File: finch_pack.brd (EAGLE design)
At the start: 14.6 x 28.3 mm, 5 parts

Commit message: board file
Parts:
- FHM-02PGR: device fujikura-fhm:FHM-02PG -> fujikura-fhm:FHM-02PGR
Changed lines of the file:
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@@
 </autorouter>
 <elements>
-<element name="FHM-02PGR" library="fujikura-fhm" package="FHM-02PG" value="FHM-02PGR" x="7.482109375" y="19.67463125" smashed="yes">
+<element name="FHM-02PGR" library="fujikura-fhm" package="FHM-02PGR" value="FHM-02PGR" x="7.482109375" y="19.67463125" smashed="yes">
 <attribute name="NAME" x="4.8442" y="16.611578125" size="0.254" layer="32" display="off"/>
 <attribute name="VALUE" x="5.80945625" y="17.18913125" size="0.4064" layer="21"/>

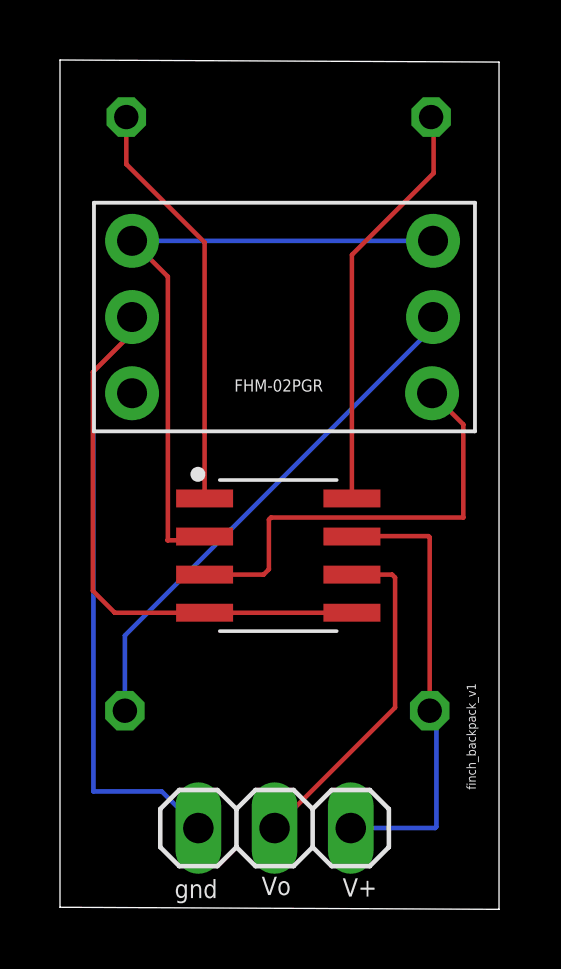
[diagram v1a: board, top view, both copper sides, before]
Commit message: board file
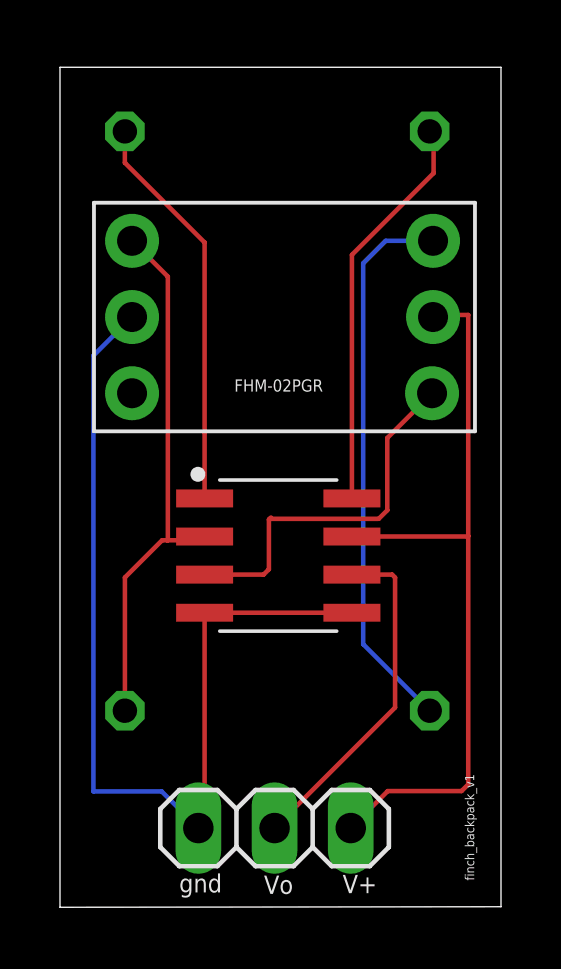
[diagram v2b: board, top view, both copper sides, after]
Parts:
- moved R1 0.48 mm to (7.24, 25.9)
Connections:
- removed net N$4: FHM-02PGR.2, R2.2
- new net N$3: FHM-02PGR.1, R2.1
- net N$2: now also R2.2; no longer FHM-02PGR.1
- net V+: now also FHM-02PGR.2; no longer R2.1
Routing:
- net N$3: track 0.00 -> 18.5 mm
- net N$4: track 17.4 -> 0.00 mm
- net V+: track 15.0 -> 25.3 mm
- net GND: track 39.0 -> 32.5 mm
- net N$2: track 21.8 -> 18.1 mm
- net N$1: track 15.0 -> 12.5 mm
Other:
- board size 14.6 x 28.3 mm -> 14.7 x 28 mm
